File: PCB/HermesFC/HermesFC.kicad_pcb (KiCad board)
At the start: 4 copper layers, 51.4 x 51.3 mm, 68 parts, among them J1 Conn_01x04, J2 Screw_Terminal_01x02, J3 Conn_01x04, J4 Conn_01x04, J5 Conn_01x04, J6 Conn_01x06, J7 USB_B_Micro, Q1 AO3401A, U1 STM32F405RGTx, U2 AP63203WU, U3 USBLC6-2SC6, U4 MPU-6050, U5 ICM-20948, U6 LD39015M18R, U7 NTS0104PW, U8 BMP280, Y1 16Mhz

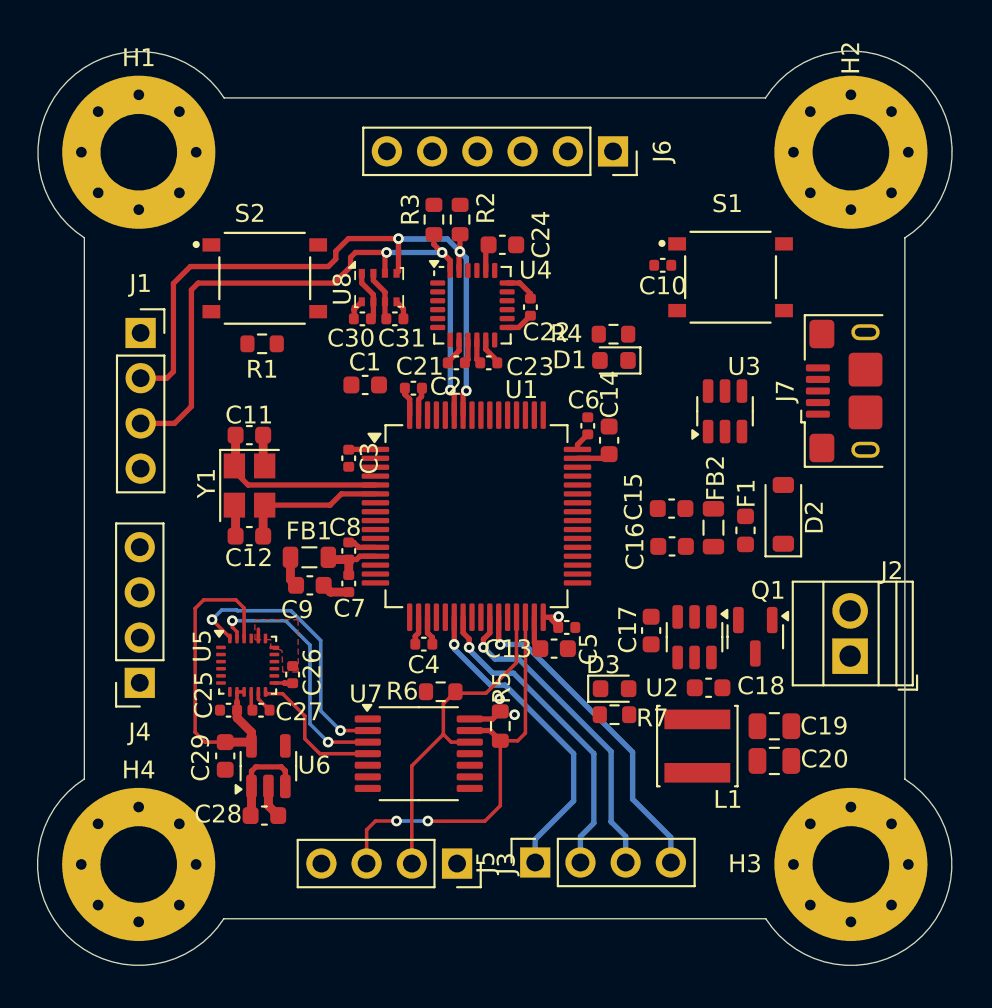
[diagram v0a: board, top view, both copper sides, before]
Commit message: complete compact routing
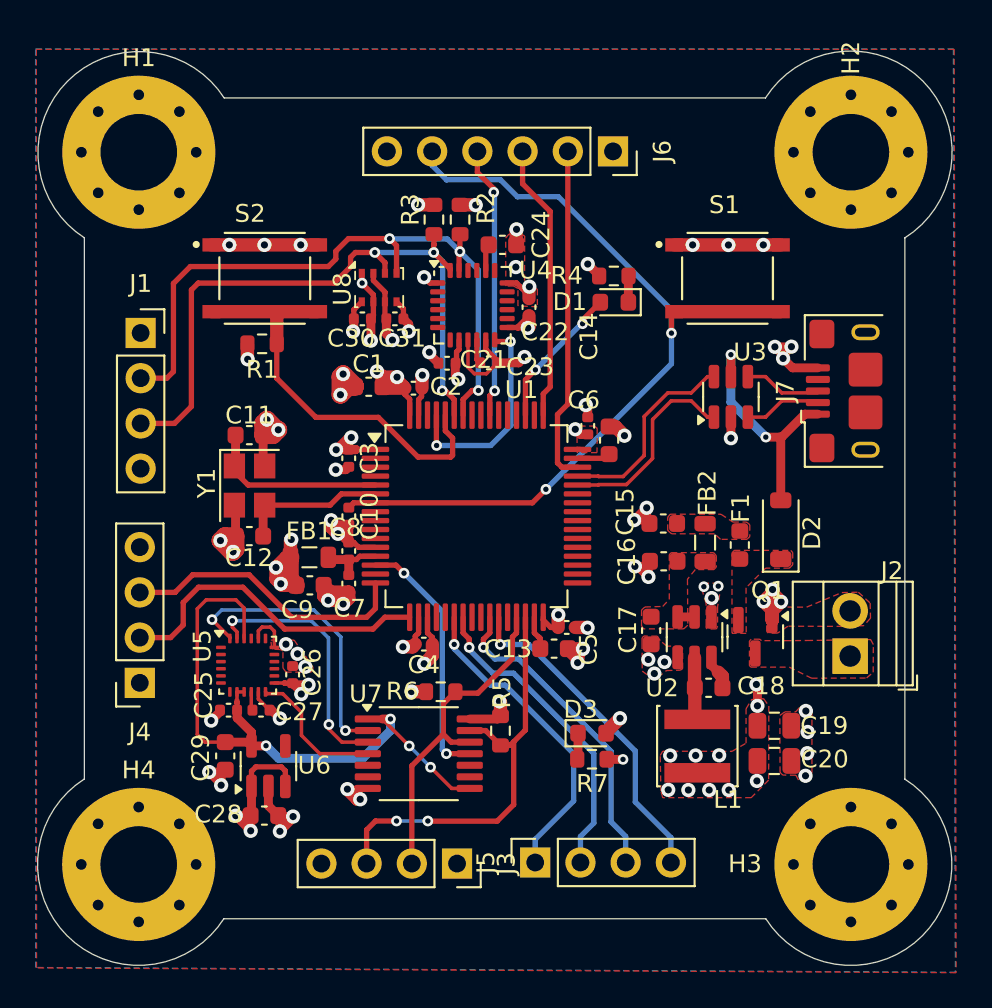
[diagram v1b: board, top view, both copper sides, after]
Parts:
- moved C10 22.6 mm to (122.9, 98.5), turned to -90 degrees
- moved D1 3.27 mm to (137.8, 86.5)
- moved R4 3.27 mm to (137.8, 85.0)
- moved D3 2.80 mm to (136.5, 110.7)
- moved R7 2.80 mm to (136.5, 112.1)
- moved C15 0.96 mm to (140.5, 98.9)
- moved C16 0.96 mm to (140.6, 101.0)
- moved FB2 0.96 mm to (142.9, 100.0)
- moved F1 0.88 mm to (144.8, 100.1)
- moved U3 0.87 mm to (144.3, 91.8)
- moved D2 0.87 mm to (147.1, 99.2)
- moved C21 0.52 mm to (128.4, 89.9), turned to 0 degrees
- moved R5 0.26 mm to (131.4, 110.5)
- moved C1 0.22 mm to (124.0, 91.2)
- moved S1 0.18 mm to (144.1, 85.1)
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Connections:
- H1 pad 1: (no net) -> GND
- H2 pad 1: (no net) -> GND
- H3 pad 1: (no net) -> GND
- H4 pad 1: (no net) -> GND
- J6 pad 2: SWCLK -> SWDIO
- J6 pad 3: SWDIO -> SWCLK
- U1 pad 51: unconnected-(U1-PC10-Pad51) -> LED
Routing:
- net GND: track 22.3 -> 94.0 mm, vias 0 -> 62
- net /STM32/NRST: track 0.00 -> 49.4 mm, vias 0 -> 2
- net +3V3: track 24.3 -> 58.4 mm, vias 3 -> 39
- net /STM32/BOOT0: track 0.00 -> 23.9 mm
- net SWDIO: track 0.00 -> 19.0 mm
- net USART2_RX: track 0.00 -> 18.3 mm
- net VDDIO_1v8: track 19.1 -> 36.1 mm, vias 0 -> 4
- net USART2_TX: track 0.00 -> 16.3 mm
- net SWCLK: track 0.00 -> 15.6 mm
- net SWO: track 0.00 -> 15.3 mm, vias 0 -> 2
- net ICM_INT_3v3: track 0.00 -> 14.2 mm, vias 0 -> 2
- net +5V: track 0.00 -> 13.7 mm, vias 0 -> 2
- net IMU_INT: track 0.00 -> 12.0 mm, vias 0 -> 2
- net USB_D+: track 0.00 -> 11.3 mm
- net USB_D-: track 0.00 -> 11.3 mm
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- added copper zone on F.Cu, net +12V
- added copper zone on B.Cu, net +3V3
- added copper zone on F.Cu, net +3V3
- added copper zone on F.Cu, net /STM32/BUCK_IN
- added copper zone on F.Cu, net Net-(C15-Pad1)
- added copper zone on F.Cu, net Net-(D2-K)
